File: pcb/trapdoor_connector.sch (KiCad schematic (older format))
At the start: 1 part, among them X1 A1200_trapdoor_connector

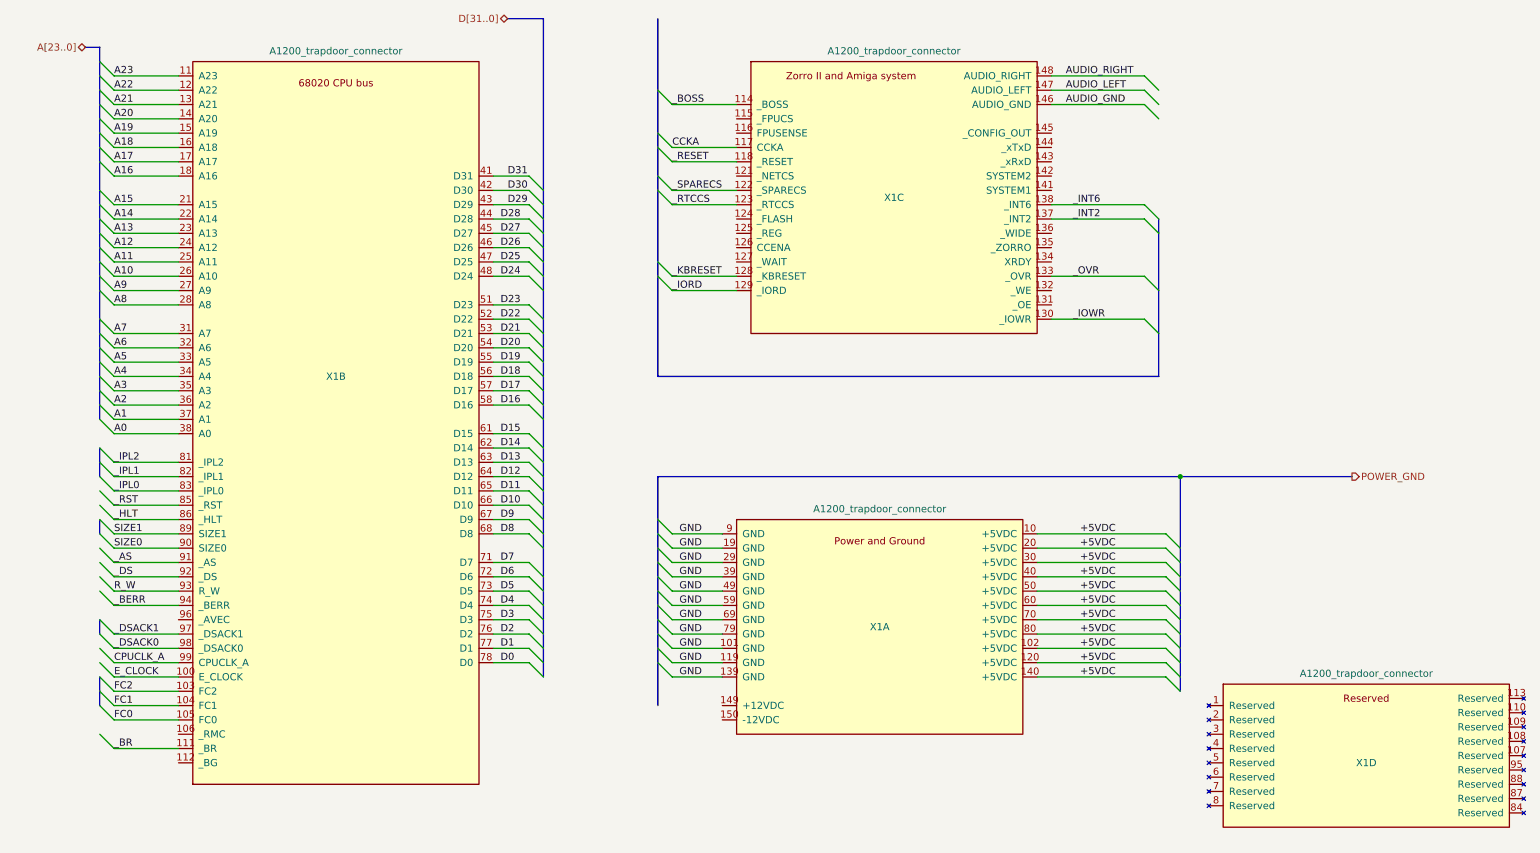
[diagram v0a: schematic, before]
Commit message: wip commit (sync work between pc's)
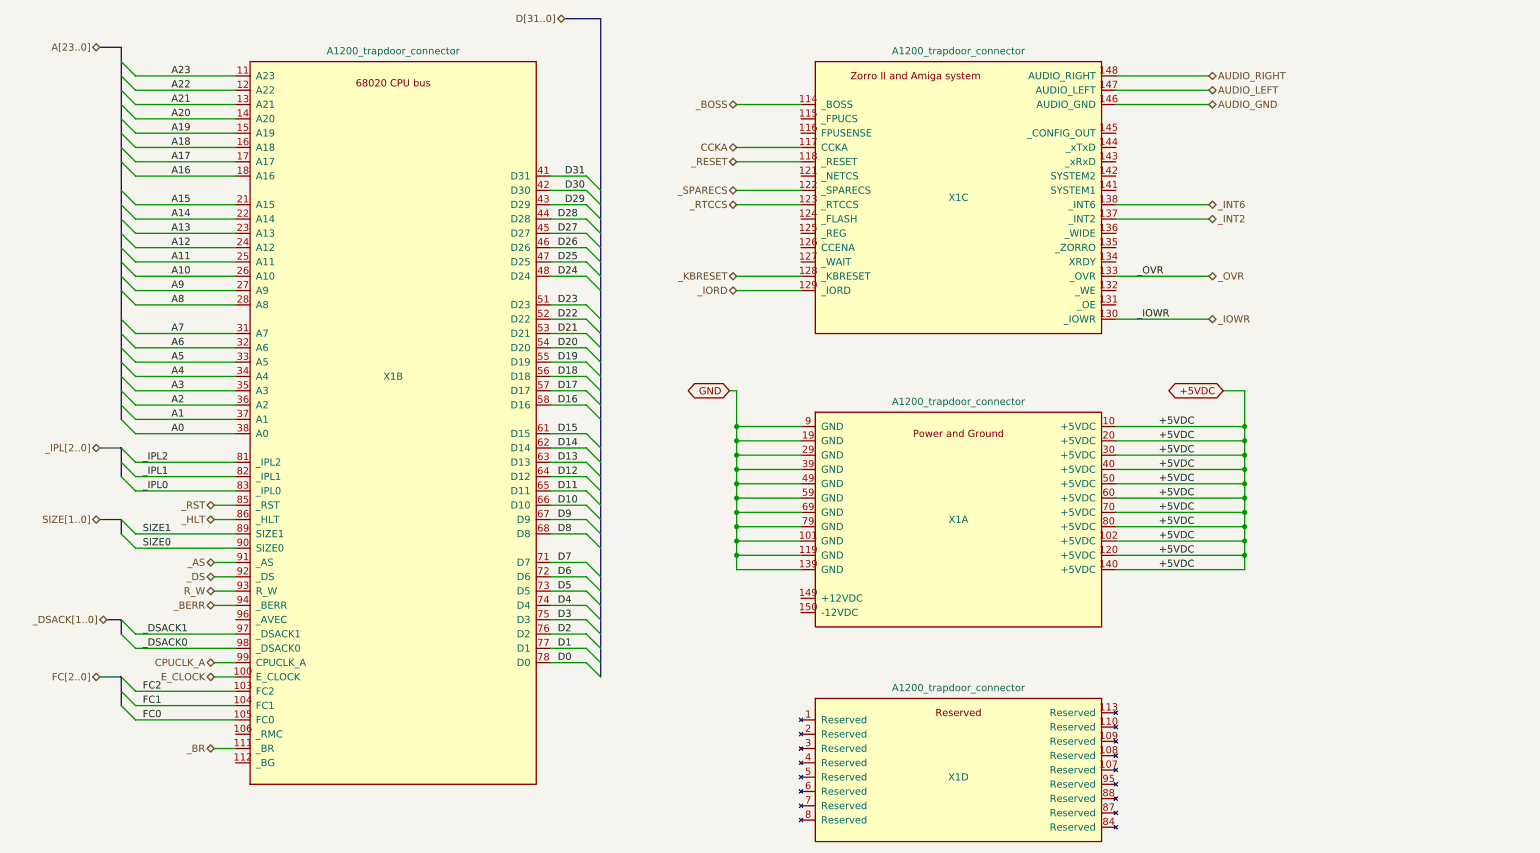
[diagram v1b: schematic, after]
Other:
- moved on the sheet: X1A, X1B, X1C, X1D
